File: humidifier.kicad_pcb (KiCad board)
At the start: 2 copper layers, 39 x 24 mm, 12 parts, among them J1 Level, J2 PWR, Q1 IRF740, U1 NE555

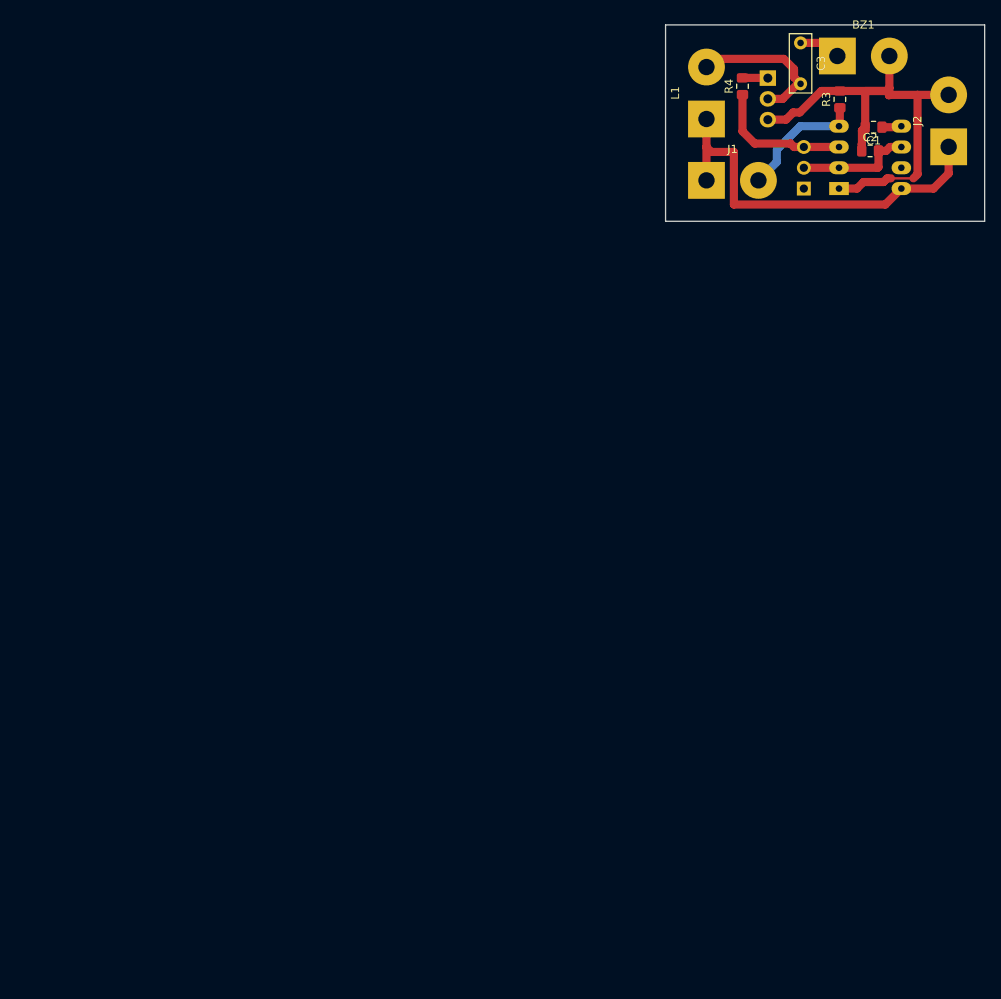
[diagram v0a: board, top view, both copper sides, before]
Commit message: Release candidate.
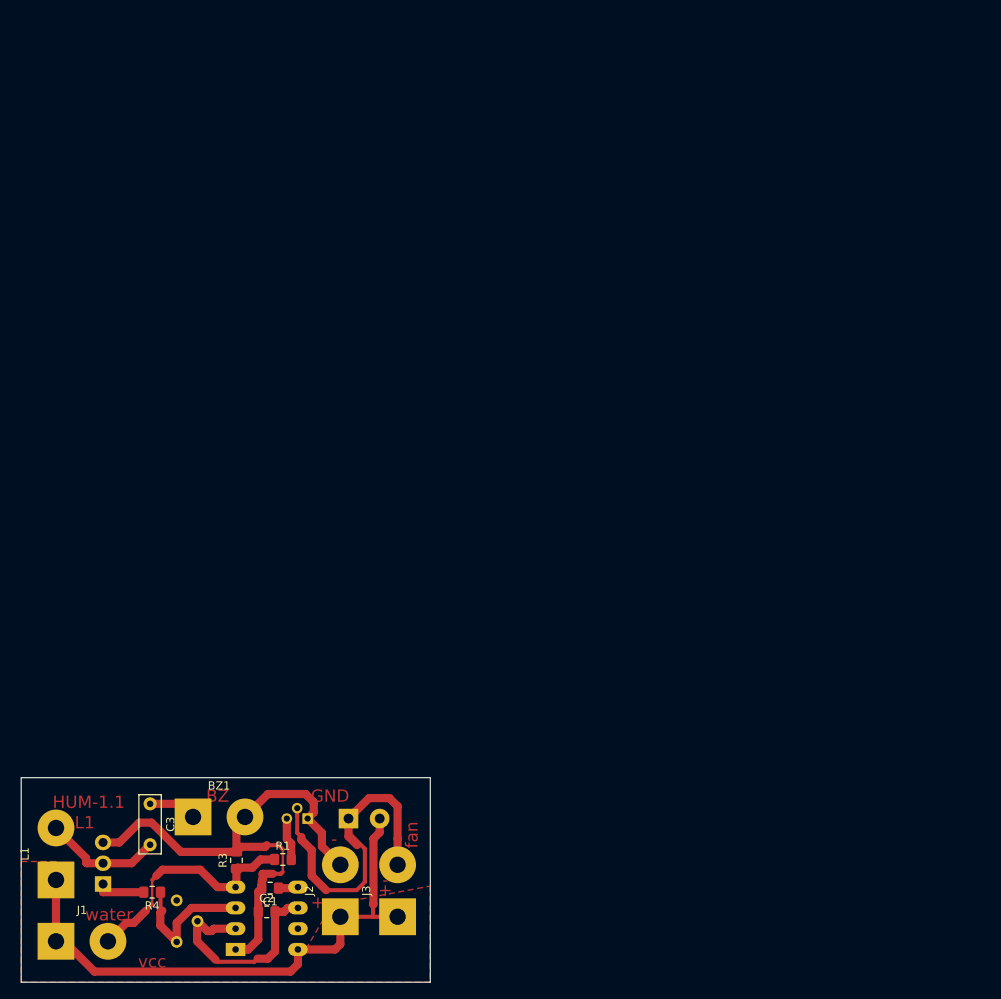
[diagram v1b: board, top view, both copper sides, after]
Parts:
- added D1: 4141, Diode_THT:D_DO-15_P3.81mm_Vertical_AnodeUp, B.Cu at (101.2, 88.0)
- added J3: FAN, Connector_Wire:SolderWirePad_1x02_P7.62mm_Drill2mm, F.Cu at (107.2, 100.0)
- added Q2: 13001, Package_TO_SOT_THT:TO-92, B.Cu at (96.2, 88.0)
- added R1: 1k, Resistor_SMD:R_0805_2012Metric_Pad1.15x1.40mm_HandSolder, F.Cu at (93.2, 93.0)
- RV1: footprint Connector_PinSocket_2.54mm:PinSocket_1x03_P2.54mm_Vertical -> Potentiometer_THT:Potentiometer_Bourns_3386P_Vertical
- moved Q1 127.7 mm to (71.2, 96.0), turned to 90 degrees
- moved C3 122.3 mm to (77.0, 86.2)
- moved J1 122.3 mm to (65.5, 103.0)
- moved L1 122.3 mm to (65.5, 95.5)
- moved R4 122.1 mm to (77.2, 97.0), turned to 180 degrees
- moved BZ1 121.9 mm to (82.2, 87.8)
- moved J2 119.9 mm to (100.2, 100.0)
- moved C1 118.7 mm to (91.7, 96.5)
- moved R3 118.7 mm to (87.5, 93.1)
- moved U1 118.7 mm to (87.4, 104.0)
- moved C2 118.7 mm to (91.2, 99.4)
- moved RV1 115.9 mm to (80.2, 98.0)
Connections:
- net Net-(J1-Pad2) renamed water
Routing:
- net Net-(D1-Pad1): track 0.00 -> 43.5 mm
- net VCC: track 56.2 -> 68.9 mm
- net 26: track 14.1 -> 26.7 mm
- net water: track 17.4 -> 29.3 mm
- net GND: track 59.9 -> 66.2 mm
- net Net-(Q2-Pad3): track 0.00 -> 5.22 mm
- net Net-(C3-Pad2): track 18.5 -> 14.5 mm
- net Net-(Q1-Pad1): track 3.11 -> 5.97 mm
- net Net-(BZ1-Pad1): track 5.16 -> 5.91 mm
- added copper zone on F.Cu, net VCC
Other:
- board size 39 x 24 mm -> 50 x 25 mm
- board text added: "+"
- board text added: "-"
- board text added: "BZ"
- board text added: "GND"
- board text added: "HUM-1.1"
- board text added: "L1"
- board text added: "fan"
- board text added: "vcc"
- board text added: "water"
